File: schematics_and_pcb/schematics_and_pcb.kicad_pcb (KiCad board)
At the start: 2 copper layers, 61.8 x 89.9 mm, 82 parts, among them J1 RND 205-00624, J2 RND 205-00627, J3 Motor con, J4 Conn_01x04_Male, J5 Conn_01x04_Male, J6 USB_OTG_custom, J7 i2c header, J8 i2c header, Q1 TSM2308CX RFG, SW1 RND 210-00210, SW2 SW_Push, U1 LP2985IM5-2.0/NOPB, U10 RND 135-00249, U11 RND 135-00249, U12 RND 135-00249, U2 TS3480CX33 RFG, U3 PWM3389DM-T3QU, U4 STM32F401RBTx, U5 LFXTAL055951, U6 9DB403DGLFT, U7 RND 135-00249, U8 RND 135-00249, U9 RND 135-00249

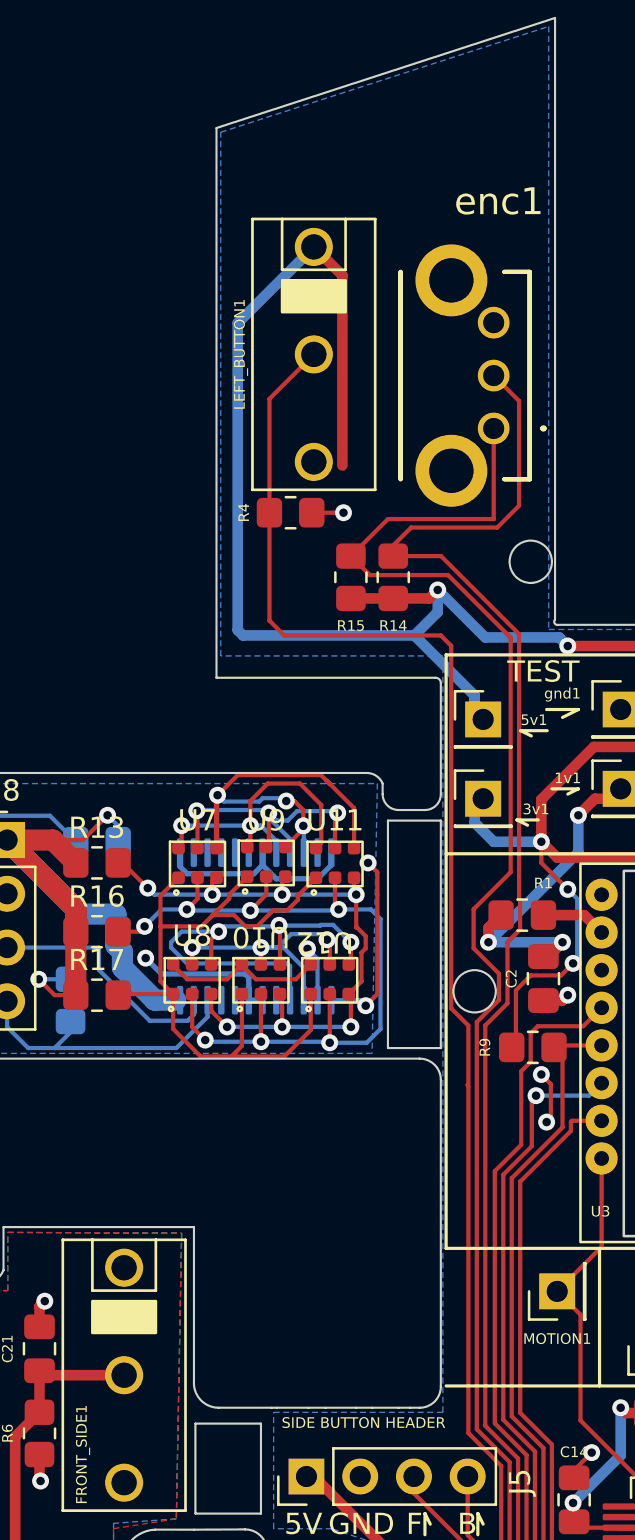
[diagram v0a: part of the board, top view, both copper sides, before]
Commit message: updated the bom
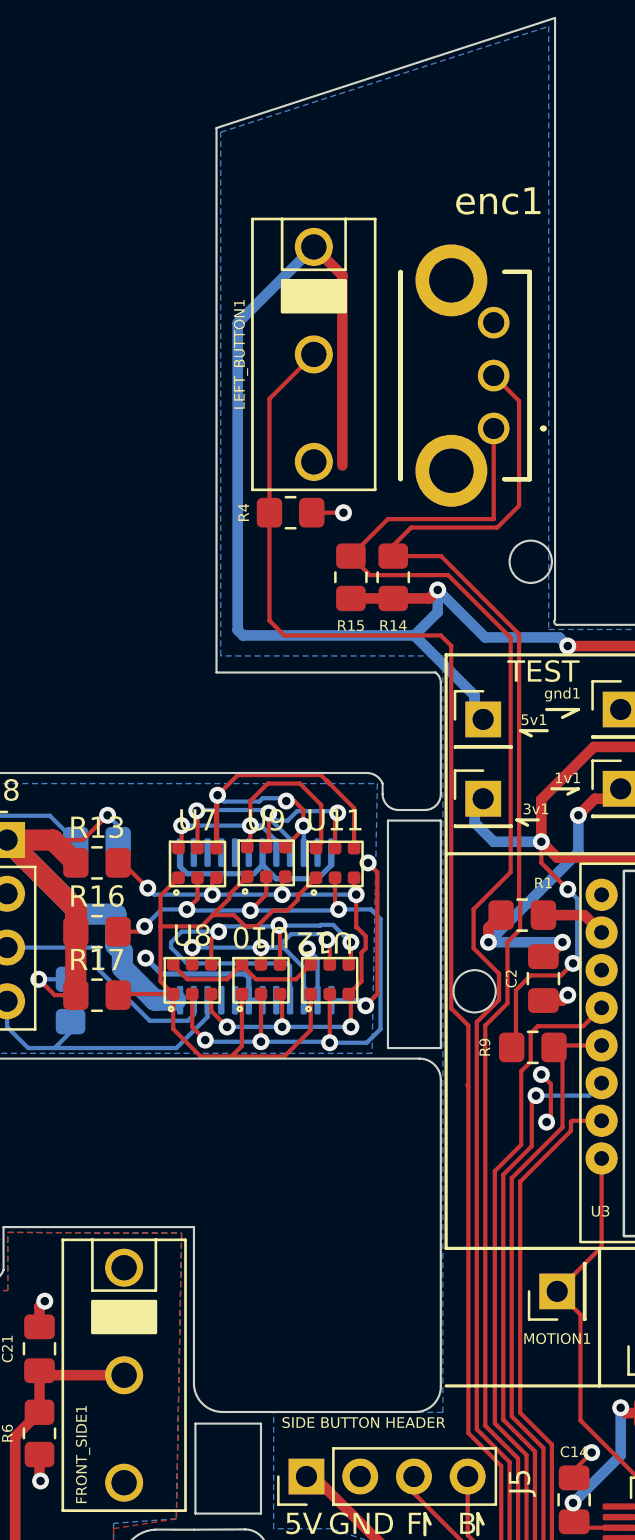
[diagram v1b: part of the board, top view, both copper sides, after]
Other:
- outline, holes or cut-outs redrawn
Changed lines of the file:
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@@
   (gr_line (start 118.49808 105.018068) (end 118.49808 107.618068) (layer "F.SilkS") (width 0.15))
   (gr_line (start 113.45 40.961932) (end 113.45 45.48) (layer "Edge.Cuts") (width 0.1))
-  (gr_line (start 90.75 90.5) (end 92 90.5) (layer "Edge.Cuts") (width 0.1))
   (gr_line (start 113.45 37.73) (end 113.45 40.961932) (layer "Edge.Cuts") (width 0.1))
-  (gr_line (start 86 90.5) (end 86.25 90.5) (layer "Edge.Cuts") (width 0.1))
   (gr_line (start 127.84808 104.968068) (end 124.34808 103.968068) (layer "Edge.Cuts") (width 0.2))
   (gr_arc (start 84.75 96.25) (mid 85.375 96.458333) (end 85.75 97) (layer "Edge.Cuts") (width 0.1))
   (gr_arc (start 80.25 100.1625) (mid 79.256047 99.768909) (end 78.9325 98.75) (layer "Edge.Cuts") (width 0.1))
-  (gr_line (start 83.5 90.5) (end 86 90.5) (layer "Edge.Cuts") (width 0.1))
-  (gr_line (start 88.55 90.5) (end 90 90.5) (layer "Edge.Cuts") (width 0.1))
+  (gr_line (start 83.75 90.7) (end 86.25 90.7) (layer "Edge.Cuts") (width 0.1))
   (gr_arc (start 90.5 60.5) (mid 90.950694 60.636459) (end 91.25 61) (layer "Edge.Cuts") (width 0.1))
   (gr_line (start 85.84808 103.75) (end 83 103.75) (layer "Edge.Cuts") (width 0.1))
@@
   (gr_line (start 122.84808 114.318068) (end 127.34808 106.718068) (layer "Edge.Cuts") (width 0.1))
   (gr_line (start 82.3325 114.4625) (end 81.8325 114.4625) (layer "Edge.Cuts") (width 0.1))
-  (gr_arc (start 93.75 56) (mid 93.926777 56.073223) (end 94 56.25) (layer "Edge.Cuts") (width 0.1))
+  (gr_arc (start 93.75 55.75) (mid 93.934017 55.970491) (end 94 56.25) (layer "Edge.Cuts") (width 0.1))
   (gr_line (start 99.39808 24.818068) (end 83.39808 30.018068) (layer "Edge.Cuts") (width 0.1))
   (gr_line (start 95.14808 114.318068) (end 122.84808 114.318068) (layer "Edge.Cuts") (width 0.1))
@@
   (gr_line (start 116.25 53.25) (end 116.25 45.75) (layer "Edge.Cuts") (width 0.1))
   (gr_arc (start 99.5 53.5) (mid 99.369135 53.407576) (end 99.39808 53.25) (layer "Edge.Cuts") (width 0.1))
-  (gr_line (start 83.39808 56) (end 83.39808 30.018068) (layer "Edge.Cuts") (width 0.1))
-  (gr_line (start 92 90.5) (end 92.55 90.5) (layer "Edge.Cuts") (width 0.1))
+  (gr_line (start 83.39808 55.75) (end 83.39808 30.018068) (layer "Edge.Cuts") (width 0.1))
   (gr_line (start 116.1 24.518068) (end 130.34808 31.718068) (layer "Edge.Cuts") (width 0.1))
   (gr_line (start 94 89.5) (end 94 75) (layer "Edge.Cuts") (width 0.1))
-  (gr_line (start 86.25 90.5) (end 87.75 90.5) (layer "Edge.Cuts") (width 0.1))
+  (gr_line (start 86.25 90.7) (end 87.75 90.7) (layer "Edge.Cuts") (width 0.1))
   (gr_line (start 82.3325 114.318068) (end 82.3325 113.5) (layer "Edge.Cuts") (width 0.1))
   (gr_circle (center 116.995316 106.318068) (end 117.995316 106.318068) (layer "Edge.Cuts") (width 0.1) (fill none))
   (gr_line (start 82.3325 89.25) (end 82.3325 81.9625) (layer "Edge.Cuts") (width 0.1))
   (gr_circle (center 107.09808 112.418068) (end 108.09808 112.418068) (layer "Edge.Cuts") (width 0.1) (fill none))
-  (gr_arc (start 94 89.5) (mid 93.707107 90.207107) (end 93 90.5) (layer "Edge.Cuts") (width 0.1))
+  (gr_arc (start 94 89.5) (mid 93.630731 90.366386) (end 92.75 90.7) (layer "Edge.Cuts") (width 0.1))
   (gr_arc (start 116 45.5) (mid 116.176777 45.573223) (end 116.25 45.75) (layer "Edge.Cuts") (width 0.1))
   (gr_line (start 80.0325 114.4625) (end 77.8325 114.4625) (layer "Edge.Cuts") (width 0.1))
@@
   (gr_line (start 115.75 37.73) (end 113.45 37.73) (layer "Edge.Cuts") (width 0.1))
   (gr_line (start 99.39808 24.818068) (end 99.39808 53.25) (layer "Edge.Cuts") (width 0.1))
-  (gr_line (start 93 90.5) (end 92.55 90.5) (layer "Edge.Cuts") (width 0.1))
   (gr_line (start 82.3325 81.9625) (end 73.3325 81.9625) (layer "Edge.Cuts") (width 0.1))
   (gr_rect (start 85.84808 112.75) (end 82.5 104.25) (layer "Edge.Cuts") (width 0.1) (fill none))
@@
   (gr_arc (start 116.25 53.25) (mid 116.176777 53.426777) (end 116 53.5) (layer "Edge.Cuts") (width 0.1))
   (gr_line (start 68.5325 84.6625) (end 68.5325 111.7625) (layer "Edge.Cuts") (width 0.1))
-  (gr_line (start 87.75 90.5) (end 88.55 90.5) (layer "Edge.Cuts") (width 0.1))
   (gr_line (start 93.25 62.25) (end 92 62.25) (layer "Edge.Cuts") (width 0.1))
   (gr_line (start 91.25 61) (end 91.25 61.5) (layer "Edge.Cuts") (width 0.1))
+  (gr_line (start 87.75 90.7) (end 92.75 90.7) (layer "Edge.Cuts") (width 0.1))
   (gr_line (start 130.34808 50.818068) (end 130.34808 91.718068) (layer "Edge.Cuts") (width 0.1))
   (gr_line (start 85.5 113.25) (end 82.5 113.25) (layer "Edge.Cuts") (width 0.1))
@@
   (gr_line (start 78.9325 98.75) (end 78.9325 97.75) (layer "Edge.Cuts") (width 0.1))
   (gr_line (start 129.82808 97.288068) (end 130.34808 91.718068) (layer "Edge.Cuts") (width 0.1))
-  (gr_arc (start 83.5 90.5) (mid 82.644787 90.128546) (end 82.3325 89.25) (layer "Edge.Cuts") (width 0.1))
+  (gr_arc (start 83.75 90.7) (mid 82.716488 90.292482) (end 82.3325 89.25) (layer "Edge.Cuts") (width 0.1))
   (gr_line (start 80.5 96.259835) (end 82.3325 96.2625) (layer "Edge.Cuts") (width 0.1))
   (gr_line (start 99.5 53.5) (end 116 53.5) (layer "Edge.Cuts") (width 0.1))
@@
   (gr_line (start 80.0325 114.4625) (end 81.8325 114.4625) (layer "Edge.Cuts") (width 0.1))
   (gr_line (start 85.75 97) (end 89.34808 97.018068) (layer "Edge.Cuts") (width 0.1))
-  (gr_line (start 83.39808 56) (end 93.75 56) (layer "Edge.Cuts") (width 0.1))
+  (gr_line (start 83.39808 55.75) (end 93.75 55.75) (layer "Edge.Cuts") (width 0.1))
   (gr_line (start 71.25 60.5) (end 71.25 74) (layer "Edge.Cuts") (width 0.1))
   (gr_arc (start 83 103.75) (mid 82.49799 103.524751) (end 82.3325 103) (layer "Edge.Cuts") (width 0.1))
@@
   (gr_arc (start 78.9325 97.75) (mid 79.437437 96.711635) (end 80.5 96.259835) (layer "Edge.Cuts") (width 0.1))
   (gr_circle (center 92.29808 110.318068) (end 95.59808 110.318068) (layer "Edge.Cuts") (width 0.1) (fill none))
-  (gr_line (start 90 90.5) (end 90.75 90.5) (layer "Edge.Cuts") (width 0.1))
   (gr_text "SDA\n" (at 76 69) (layer "B.SilkS")
     (effects (font (size 0.75 0.75) (thickness 0.15)) (justify mirror))
